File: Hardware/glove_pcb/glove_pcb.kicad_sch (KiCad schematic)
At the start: 0 parts

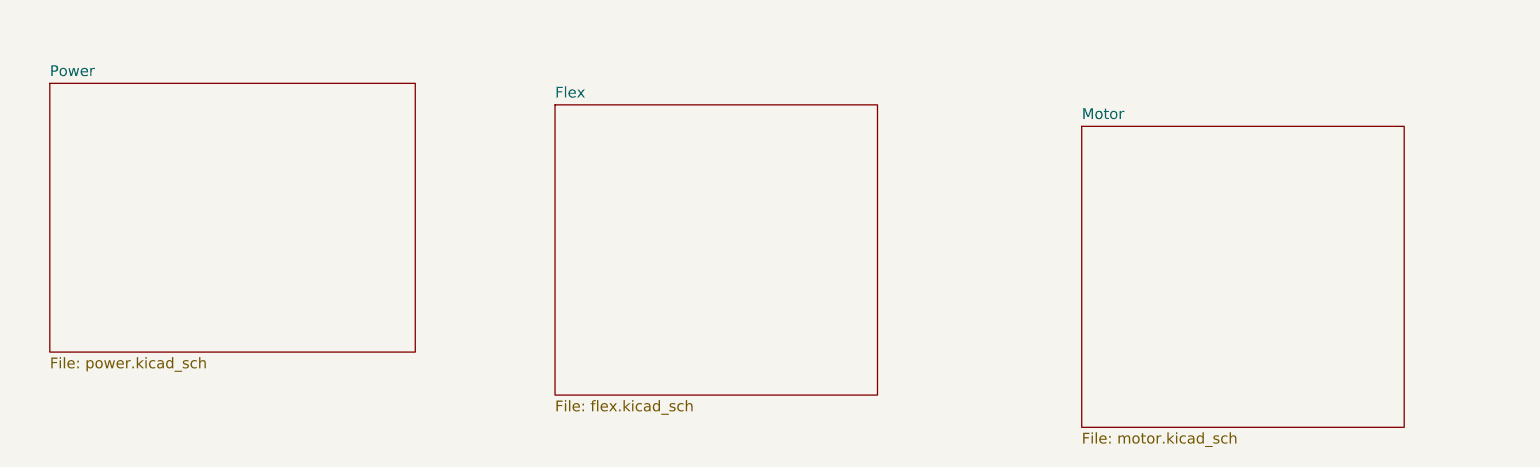
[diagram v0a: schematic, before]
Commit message: More work on motor driver connection
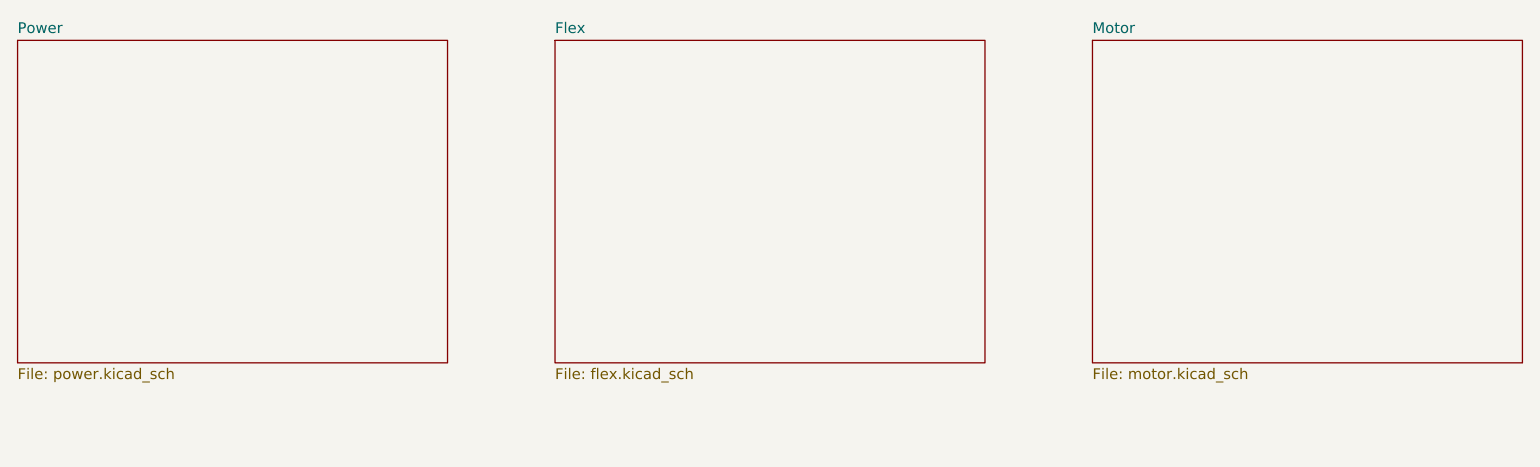
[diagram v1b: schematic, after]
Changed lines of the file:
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@@
 (kicad_sch (version 20230121) (generator eeschema)
   (paper "A4")
-  (sheet (at 54.61 55.88) (size 43.18 31.75) (fields_autoplaced)
+  (sheet (at 50.8 50.8) (size 50.8 38.1) (fields_autoplaced)
     (stroke (width 0.1524) (type solid))
     (fill (color 0 0 0 0.0000))
-    (property "Sheetname" "Power" (at 54.61 55.1684 0)
+    (property "Sheetname" "Power" (at 50.8 50.0884 0)
       (effects (font (size 1.27 1.27)) (justify left bottom))
     )
-    (property "Sheetfile" "power.kicad_sch" (at 54.61 88.2146 0)
+    (property "Sheetfile" "power.kicad_sch" (at 50.8 89.4846 0)
       (effects (font (size 1.27 1.27)) (justify left top))
     )
@@
     )
   )
-  (sheet (at 114.3 58.42) (size 38.1 34.29) (fields_autoplaced)
+  (sheet (at 114.3 50.8) (size 50.8 38.1) (fields_autoplaced)
     (stroke (width 0.1524) (type solid))
     (fill (color 0 0 0 0.0000))
-    (property "Sheetname" "Flex" (at 114.3 57.7084 0)
+    (property "Sheetname" "Flex" (at 114.3 50.0884 0)
       (effects (font (size 1.27 1.27)) (justify left bottom))
     )
-    (property "Sheetfile" "flex.kicad_sch" (at 114.3 93.2946 0)
+    (property "Sheetfile" "flex.kicad_sch" (at 114.3 89.4846 0)
       (effects (font (size 1.27 1.27)) (justify left top))
     )
@@
     )
   )
-  (sheet (at 176.53 60.96) (size 38.1 35.56) (fields_autoplaced)
+  (sheet (at 177.8 50.8) (size 50.8 38.1) (fields_autoplaced)
     (stroke (width 0.1524) (type solid))
     (fill (color 0 0 0 0.0000))
-    (property "Sheetname" "Motor" (at 176.53 60.2484 0)
+    (property "Sheetname" "Motor" (at 177.8 50.0884 0)
       (effects (font (size 1.27 1.27)) (justify left bottom))
     )
-    (property "Sheetfile" "motor.kicad_sch" (at 176.53 97.1046 0)
+    (property "Sheetfile" "motor.kicad_sch" (at 177.8 89.4846 0)
       (effects (font (size 1.27 1.27)) (justify left top))
     )
